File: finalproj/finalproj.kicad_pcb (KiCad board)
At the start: 2 copper layers, 83 parts, among them J1 Conn_01x01, J10 MotorA Out, J11 MotorB Out, J2 Conn_01x01, J3 Conn_01x01, J4 Programmer_Conn, J5 Stepper_Motor_Controller, J6 Conn_01x01, J7 LIDAR_Connector, J9 RPI_UART_Conn, SW3 SW_Push, U5 L298N, U7 STM32F401RCTx, Y1 25 MHz, Y2 32.768 KHz

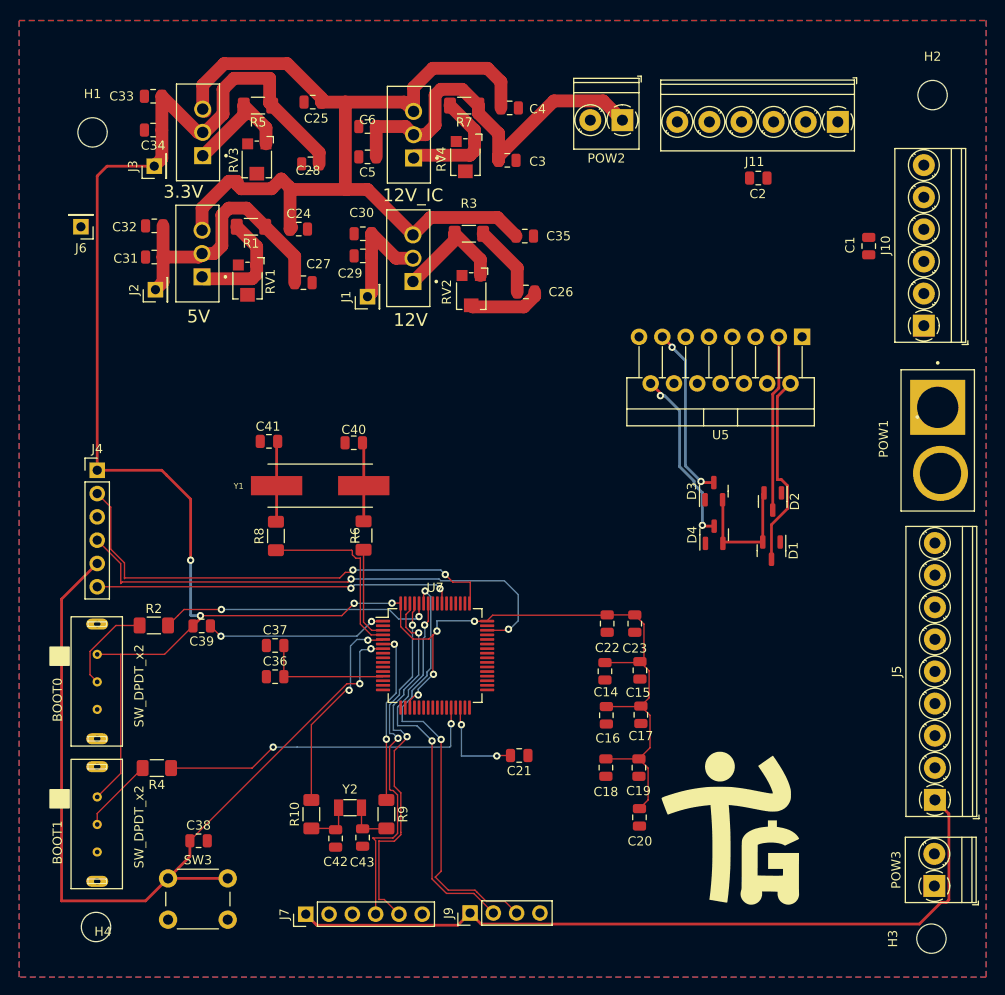
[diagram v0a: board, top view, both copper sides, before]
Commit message: jlcboard2 ready for review
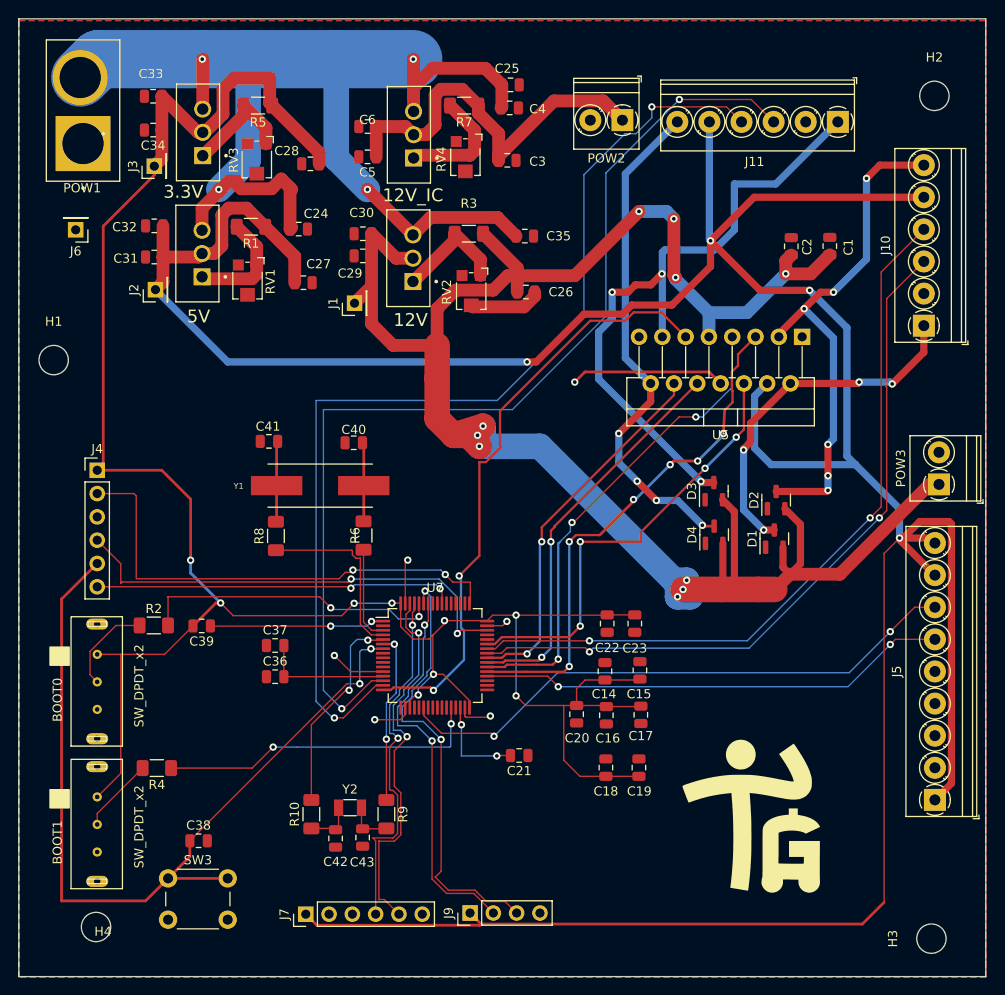
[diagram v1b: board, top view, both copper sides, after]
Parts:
- moved POW1 99.9 mm to (15.6, 15.4), turned to 90 degrees
- moved POW3 43.8 mm to (108.9, 56.1)
- moved H1 25.2 mm to (12.4, 42.6)
- moved C25 21.6 mm to (62.2, 12.6), turned to 0 degrees
- moved C20 13.2 mm to (69.4, 81.2)
- moved C2 8.26 mm to (92.8, 30.2), turned to 90 degrees
- moved C1 4.24 mm to (97.0, 30.2), turned to 90 degrees
- moved G*** 2.62 mm to (90.0, 92.8)
- moved J1 1.58 mm to (45.2, 36.4)
- moved D1 1.34 mm to (91.0, 62.1), turned to 90 degrees
- moved J6 0.66 mm to (14.8, 28.4)
- moved D2 0.40 mm to (91.2, 57.9), turned to 90 degrees
- moved H2 0.21 mm to (108.4, 13.8)
- turned C14 to -90 degrees
- turned C15 to -90 degrees
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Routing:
- net EXT_5: track 115.1 -> 357.2 mm, vias 0 -> 4
- net EXT_12: track 35.1 -> 216.4 mm, vias 0 -> 10
- net EncoderBFeedback1: track 0.00 -> 112.4 mm, vias 0 -> 2
- net EncoderBFeedback2: track 0.00 -> 112.2 mm, vias 0 -> 2
- net EncoderAFeedback2: track 0.00 -> 81.5 mm, vias 0 -> 2
- net EncoderAFeedback1: track 0.00 -> 79.3 mm, vias 0 -> 2
- net MotorBPWM: track 0.00 -> 65.8 mm, vias 0 -> 2
- net STEP_PWM: track 0.00 -> 63.3 mm, vias 0 -> 2
- net MotorAIn1: track 0.00 -> 56.5 mm, vias 0 -> 6
- net MotorAIn2: track 0.00 -> 52.7 mm, vias 0 -> 3
- net MotorOutB1: track 19.0 -> 70.7 mm, vias 2 -> 3
- net STEP_DIR: track 0.00 -> 51.4 mm, vias 0 -> 2
- net MotorAPWM: track 0.00 -> 48.7 mm, vias 0 -> 4
- net MotorBIn1: track 0.00 -> 43.1 mm, vias 0 -> 2
- net MotorBIn2: track 0.00 -> 40.6 mm, vias 0 -> 2
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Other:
- board outline added: 105.4 x 104.4 mm
